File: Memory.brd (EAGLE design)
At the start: 105.4 x 56.8 mm, 4 parts, among them IC5 HM62256DIP

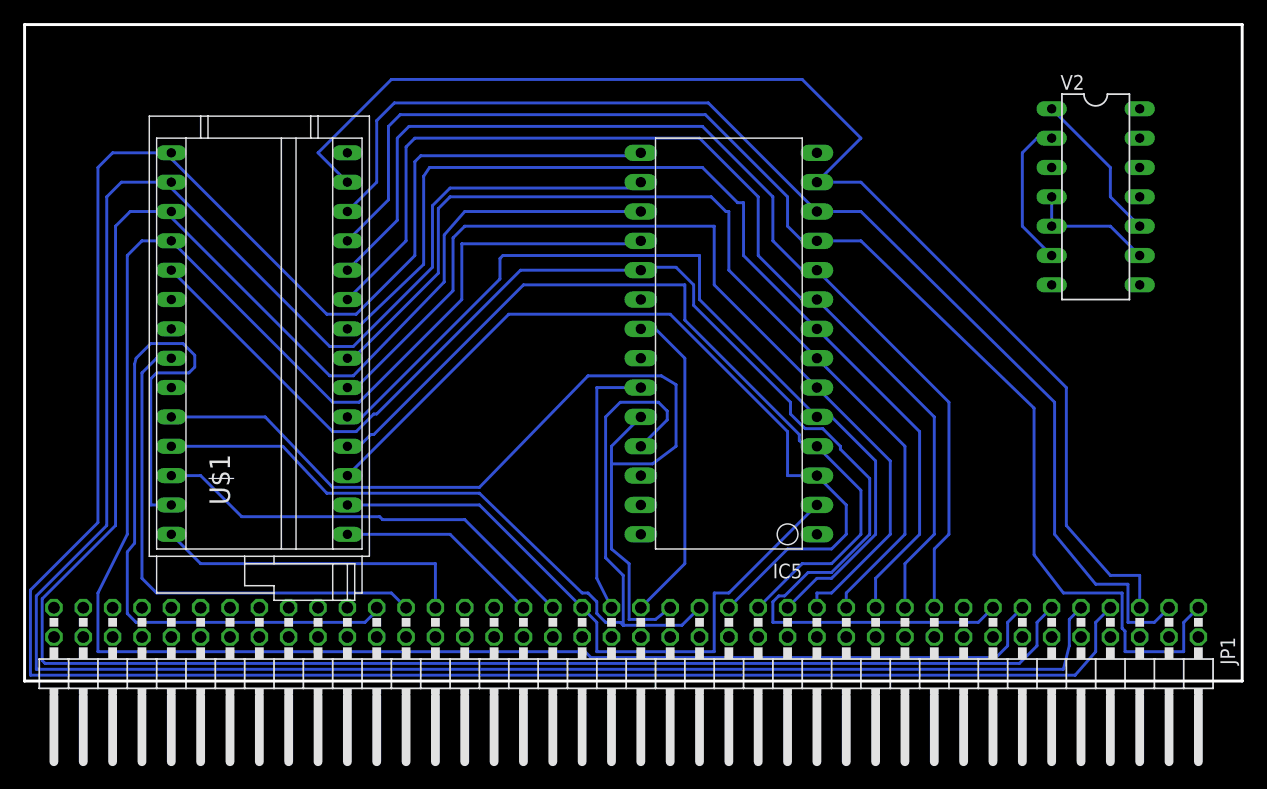
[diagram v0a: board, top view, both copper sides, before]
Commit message: Finish Modularization
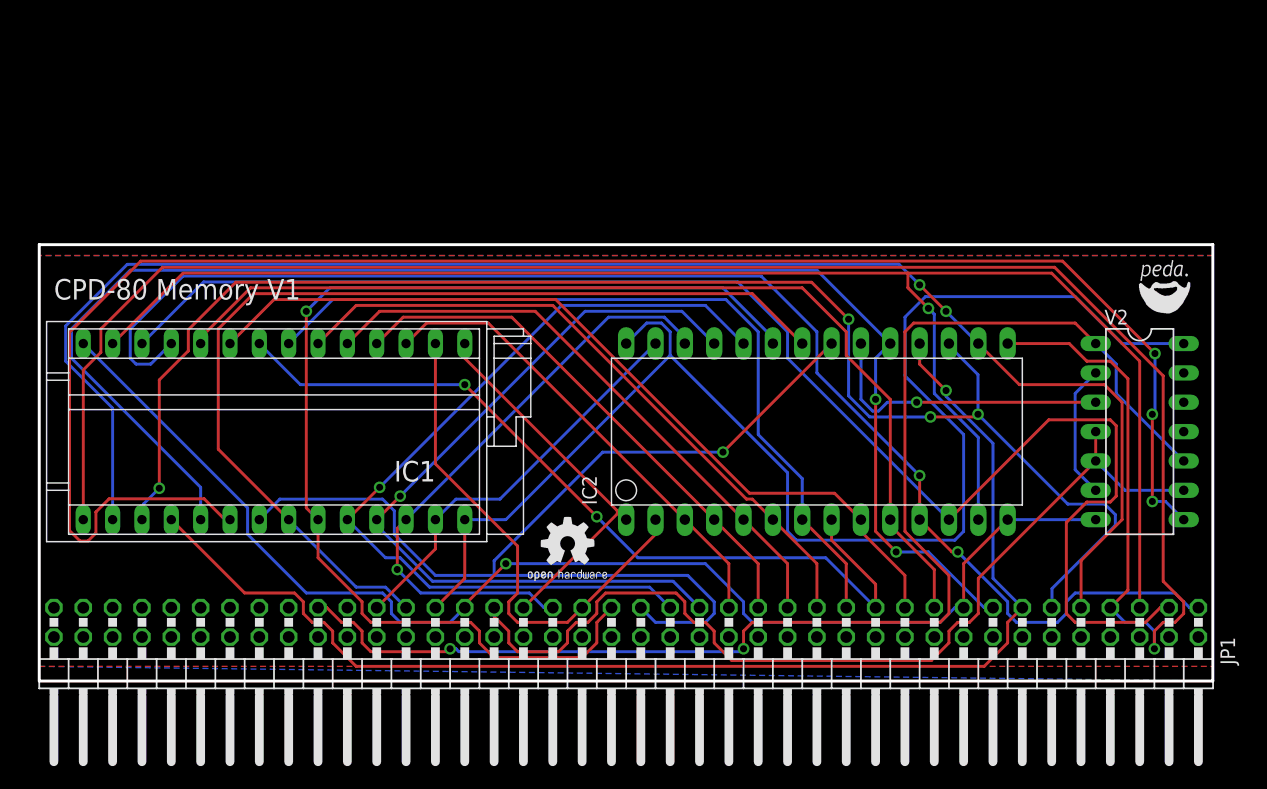
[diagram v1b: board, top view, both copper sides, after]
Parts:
- removed IC5: HM62256DIP, jean:HM62256-DIP
- added IC1: AT28C256ZIF, bt_memory:DIL28-ZIF
- added IC2: HM62256DIP, jean:HM62256-DIP
- U$1: value AT28C256ZIF -> (none); device bt_memory:DIL28-ZIF -> bfl:OSHW2
- moved U$1 31.4 mm to (43.2, 7.62), turned to 0 degrees
- moved V2 20.7 mm to (96.5, 21.6)
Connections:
- net !RD: now also IC1.22, IC2.22; no longer IC5.22, U$1.22
- net !WR: now also IC1.27, IC2.27; no longer IC5.27, U$1.27
- net A0: now also IC1.10, IC2.10; no longer IC5.10, U$1.10
- net A1: now also IC1.9, IC2.9; no longer IC5.9, U$1.9
- net A10: now also IC1.21, IC2.21; no longer IC5.21, U$1.21
- net A11: now also IC1.23, IC2.23; no longer IC5.23, U$1.23
- net A12: now also IC1.2, IC2.2; no longer IC5.2, U$1.2
- net A13: now also IC1.26, IC2.26; no longer IC5.26, U$1.26
- net A14: now also IC1.1, IC2.1; no longer IC5.1, U$1.1
- net A2: now also IC1.8, IC2.8; no longer IC5.8, U$1.8
- net A3: now also IC1.7, IC2.7; no longer IC5.7, U$1.7
- net A4: now also IC1.6, IC2.6; no longer IC5.6, U$1.6
- net A5: now also IC1.5, IC2.5; no longer IC5.5, U$1.5
- net A6: now also IC1.4, IC2.4; no longer IC5.4, U$1.4
- net A7: now also IC1.3, IC2.3; no longer IC5.3, U$1.3
- net A8: now also IC1.25, IC2.25; no longer IC5.25, U$1.25
- net A9: now also IC1.24, IC2.24; no longer IC5.24, U$1.24
- net D0: now also IC1.11, IC2.11; no longer IC5.11, U$1.11
- net D1: now also IC1.12, IC2.12; no longer IC5.12, U$1.12
- net D2: now also IC1.13, IC2.13; no longer IC5.13, U$1.13
- net D3: now also IC1.15, IC2.15; no longer IC5.15, U$1.15
- net D4: now also IC1.16, IC2.16; no longer IC5.16, U$1.16
- net D5: now also IC1.17, IC2.17; no longer IC5.17, U$1.17
- net D6: now also IC1.18, IC2.18; no longer IC5.18, U$1.18
- net D7: now also IC1.19, IC2.19; no longer IC5.19, U$1.19
- net GND: now also IC1.14, IC2.14; no longer IC5.14, U$1.14
- net N$2: now also IC1.20; no longer U$1.20
- net N$9: now also IC2.20; no longer IC5.20
- net VCC: now also IC1.28, IC2.28; no longer IC5.28, U$1.28
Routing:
- net N$2: track 0.00 -> 150.9 mm, vias 0 -> 3
- net GND: track 0.00 -> 110.4 mm, vias 0 -> 1
- net !MREQ: track 13.3 -> 116.1 mm, vias 0 -> 2
- net VCC: track 27.7 -> 121.8 mm
- net A11: track 23.2 -> 98.3 mm, vias 0 -> 1
- net A15: track 11.2 -> 82.3 mm
- net D6: track 177.5 -> 109.8 mm, vias 0 -> 1
- net D4: track 200.1 -> 136.3 mm, vias 0 -> 2
- net A10: track 28.0 -> 91.5 mm, vias 0 -> 1
- net D5: track 191.5 -> 129.9 mm, vias 0 -> 4
- net !RD: track 44.8 -> 85.9 mm
- net !WR: track 68.9 -> 35.1 mm
- net A7: track 73.4 -> 41.1 mm
- net A6: track 75.3 -> 46.6 mm
- net D3: track 208.0 -> 179.5 mm, vias 0 -> 1
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- added copper zone on layer 1, net GND
- added copper zone on layer 16, net GND
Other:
- board size 105.4 x 56.8 mm -> 101.6 x 37.8 mm
- board text added: "CPD-80 Memory V1"
